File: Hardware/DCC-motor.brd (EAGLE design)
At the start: 22.3 x 13 mm, 29 parts, among them U1 G2X[2/3]1---RSA16, U2 LP2985, U3 24LC00OT, U4 DRV8838

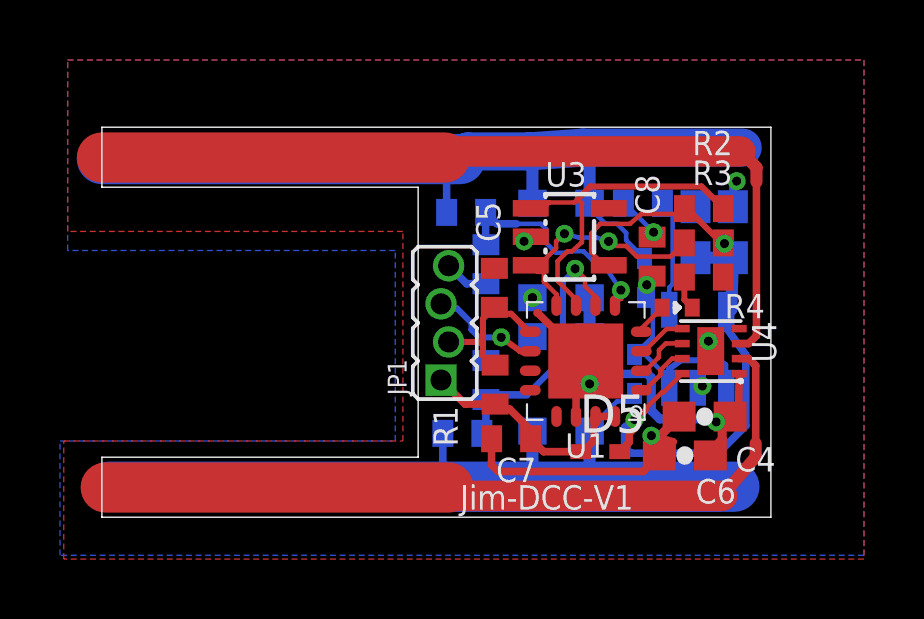
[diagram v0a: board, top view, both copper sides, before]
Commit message: Update hardware design
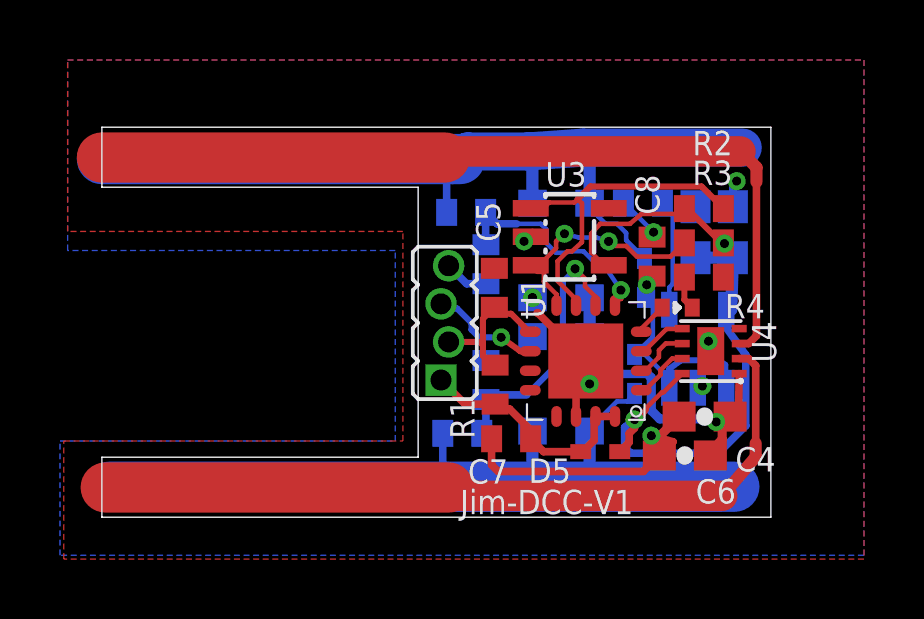
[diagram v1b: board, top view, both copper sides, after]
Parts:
- C2: value 47uF -> 0.1uF
- C3: value 47uF -> 10uF
- C7: value 0.1uF -> 47uF
- R1: value 4.7K -> 47K
- R5, R7: value 4.7K -> 9.1K
- R6, R8: value 4.7K -> 2.7K
